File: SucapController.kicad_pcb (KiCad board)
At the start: 2 copper layers, 39.2 x 30.4 mm, 46 parts, among them J1 Conn_01x14, J2 , J4 Conn_02x03_Counter_Clockwise, J5 Conn_02x03_Counter_Clockwise, J6 Conn_02x03_Counter_Clockwise, J7 Screw_Terminal_01x01, Q1 SI2301, U1 HX9193-33GB, U2 HX9193, U3 W25Q32JVSS, U4 STM32H750VBT6, U5 TL431, U6 74LVC1G17, Y1 25M, Y2 32.768K

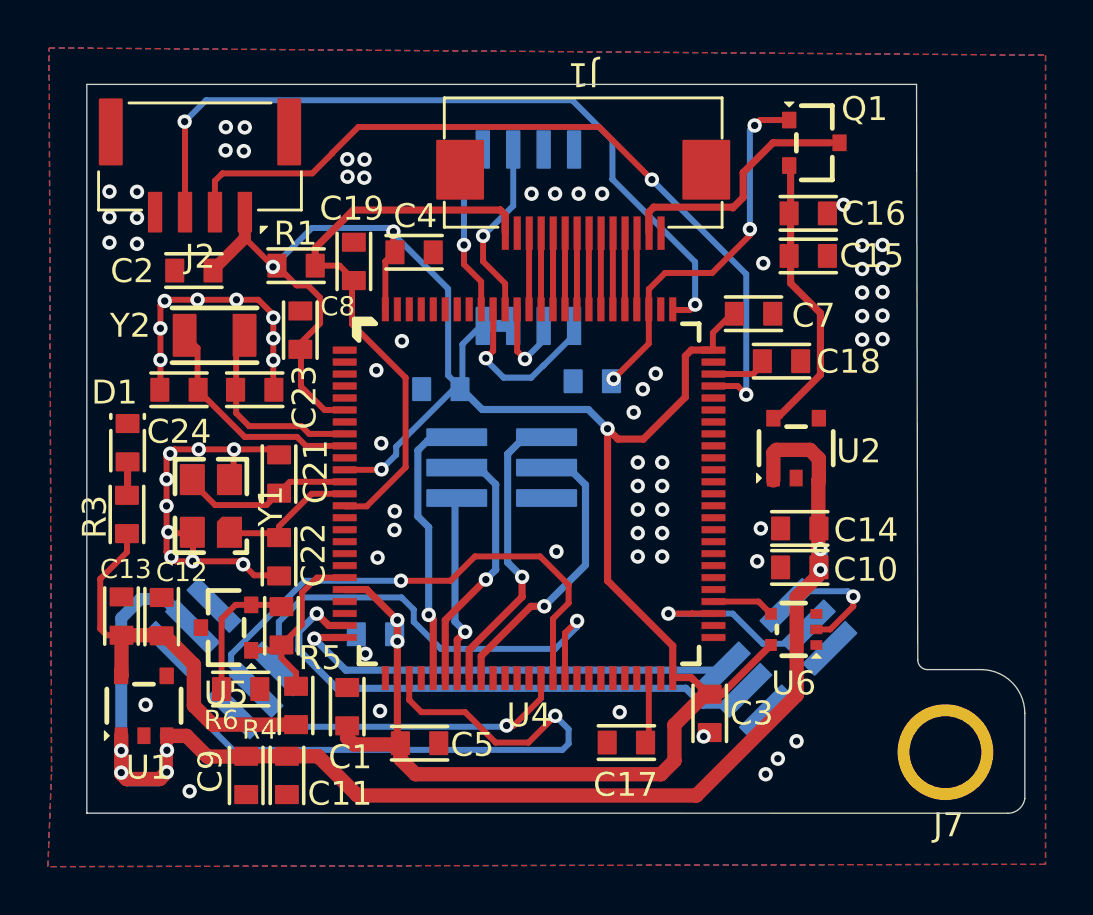
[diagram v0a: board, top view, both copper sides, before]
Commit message: fix some error
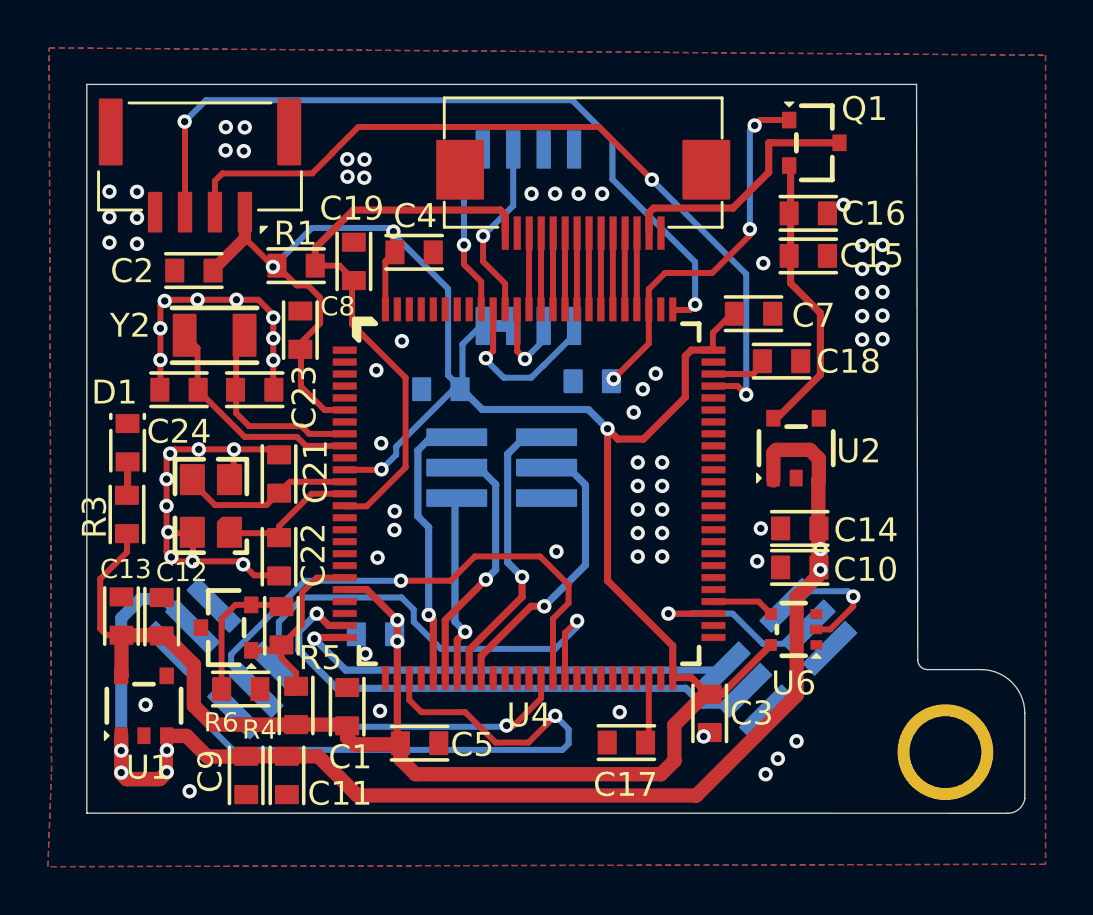
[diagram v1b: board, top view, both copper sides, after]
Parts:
-  : renamed from U5
-  : renamed from J2
-  : renamed from J1
-  : renamed from J7
-  : renamed from Y1
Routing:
- net +3V3: track 118.1 -> 120.2 mm
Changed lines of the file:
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@@
     (property "Sheetname" "")
     (attr smd)
-    (fp_text reference "U5" (at 0 2.75 unlocked) (layer "F.SilkS")
+    (fp_text reference " " (at 0 2.75 unlocked) (layer "F.SilkS")
       (effects (font (size 1 1) (thickness 0.15)))
     )
@@
     (property "Sheetname" "")
     (attr smd)
-    (fp_text reference "J2" (at 0 3.81 unlocked) (layer "F.SilkS")
+    (fp_text reference " " (at 0 3.81 unlocked) (layer "F.SilkS")
       (effects (font (size 1 1) (thickness 0.15)))
     )
@@
     (property "Sheetname" "")
     (attr smd)
-    (fp_text reference "J1" (at 0 3.683 180 unlocked) (layer "F.SilkS")
+    (fp_text reference " " (at 0 3.683 180 unlocked) (layer "F.SilkS")
       (effects (font (size 1 1) (thickness 0.15)))
     )
@@
     (property "Sheetname" "")
     (attr smd)
-    (fp_text reference "J7" (at 0 3.048 unlocked) (layer "F.SilkS")
+    (fp_text reference " " (at 0 3.048 unlocked) (layer "F.SilkS")
       (effects (font (size 1 1) (thickness 0.15)))
     )
@@
     (property "Sheetname" "")
     (attr smd)
-    (fp_text reference "Y1" (at 0 2.5 90 unlocked) (layer "F.SilkS")
+    (fp_text reference " " (at 0 2.5 90 unlocked) (layer "F.SilkS")
       (effects (font (size 1 1) (thickness 0.15)))
     )
@@
     (property "Sheetname" "")
     (attr smd)
-    (fp_text reference "R6" (at 0.8128 -1.2954) (layer "F.SilkS")
+    (fp_text reference "R6" (at 0.8128 -1.397) (layer "F.SilkS")
       (effects (font (size 0.8 0.8) (thickness 0.15)))
     )
@@
   (segment (start 212.2016 108.3184) (end 212.3948 108.3184) (width 0.6) (layer "F.Cu") (net 2))
   (segment (start 208.1276 97.2312) (end 208.561711 97.665311) (width 0.3) (layer "F.Cu") (net 2))
+  (segment (start 197.2056 109.5882) (end 197.2564 109.639) (width 0.6) (layer "F.Cu") (net 2))
   (segment (start 196.310994 96.449) (end 195.326 95.464006) (width 0.25) (layer "F.Cu") (net 2))
   (segment (start 199.479 110.363) (end 199.479 111.029) (width 0.6) (layer "F.Cu") (net 2))
@@
   (segment (start 199.479 111.029) (end 200.11 111.66) (width 0.6) (layer "F.Cu") (net 2))
   (segment (start 195.326 95.464006) (end 195.326 93.6374) (width 0.25) (layer "F.Cu") (net 2))
+  (segment (start 195.1228 109.5882) (end 197.2056 109.5882) (width 0.6) (layer "F.Cu") (net 2))
   (segment (start 187.2106 105.8544) (end 186.944 105.5878) (width 0.25) (layer "F.Cu") (net 2))
   (segment (start 198.671 98.949) (end 197.176 98.949) (width 0.25) (layer "F.Cu") (net 2))
   (segment (start 197.5358 110.4138) (end 199.4282 110.4138) (width 0.6) (layer "F.Cu") (net 2))
-  (segment (start 197.2056 109.5882) (end 197.2564 109.639) (width 0.6) (layer "F.Cu") (net 2))
   (segment (start 197.2564 110.1344) (end 197.5358 110.4138) (width 0.6) (layer "F.Cu") (net 2))
   (segment (start 199.4282 110.4138) (end 199.479 110.363) (width 0.6) (layer "F.Cu") (net 2))
@@
   (segment (start 214.2068 94.949) (end 214.617 94.5388) (width 0.25) (layer "F.Cu") (net 95))
   (segment (start 212.526 94.949) (end 214.2068 94.949) (width 0.25) (layer "F.Cu") (net 95))
-  (segment (start 213.33 87.98) (end 210.059419 87.98) (width 0.3) (layer "F.Cu") (net 96))
-  (segment (start 215.0364 85.2932) (end 213.7918 86.5378) (width 0.3) (layer "F.Cu") (net 96))
-  (segment (start 210.059419 87.98) (end 209.85 88.189419) (width 0.3) (layer "F.Cu") (net 96))
-  (segment (start 209.85 88.189419) (end 209.85 89.03) (width 0.3) (layer "F.Cu") (net 96))
-  (segment (start 213.36 88.01) (end 213.33 87.98) (width 0.3) (layer "F.Cu") (net 96))
-  (segment (start 213.7918 86.5378) (end 213.7918 87.5782) (width 0.3) (layer "F.Cu") (net 96))
-  (segment (start 217.4341 85.2932) (end 215.0364 85.2932) (width 0.3) (layer "F.Cu") (net 96))
-  (segment (start 213.7918 87.5782) (end 213.36 88.01) (width 0.3) (layer "F.Cu") (net 96))
-  (segment (start 194.4394 104.587) (end 194.5132 104.6608) (width 0.25) (layer "F.Cu") (net 98))
+  (segment (start 209.8616 88.2074) (end 210.0508 88.0182) (width 0.3) (layer "F.Cu") (net 96))
+  (segment (start 214.8586 85.2932) (end 217.8136 85.2932) (width 0.3) (layer "F.Cu") (net 96))
+  (segment (start 209.8616 89.0682) (end 209.8616 88.2074) (width 0.3) (layer "F.Cu") (net 96))
+  (segment (start 210.0508 88.0182) (end 213.367285 88.0182) (width 0.3) (layer "F.Cu") (net 96))
+  (segment (start 213.367285 88.0182) (end 214.8586 86.526885) (width 0.3) (layer "F.Cu") (net 96))
+  (segment (start 214.8586 86.526885) (end 214.8586 85.2932) (width 0.3) (layer "F.Cu") (net 96))
   (segment (start 193.2518 104.587) (end 194.4394 104.587) (width 0.25) (layer "F.Cu") (net 98))
   (segment (start 192.0114 105.1686) (end 192.593 104.587) (width 0.25) (layer "F.Cu") (net 98))
-  (segment (start 194.5894 104.737) (end 194.829 104.737) (width 0.25) (layer "F.Cu") (net 98))
   (segment (start 192.593 104.587) (end 193.2518 104.587) (width 0.25) (layer "F.Cu") (net 98))
   (segment (start 192.0114 108.1024) (end 192.0114 105.1686) (width 0.25) (layer "F.Cu") (net 98))
-  (segment (start 194.541 104.6886) (end 194.5894 104.737) (width 0.25) (layer "F.Cu") (net 98))
   (zone (net 0) (net_name "") (layers F&B.Cu) (hatch edge 0.508)
     (connect_pads (clearance 0))
